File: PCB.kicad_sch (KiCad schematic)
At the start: 34 parts, among them J1 USB_C_Receptacle_USB2.0, J2 JST - 1.00mm 4 Pin, SW72 SW_Push, SW73 SW_Push, U1 RP2040, U2 SOP-8 SPI FLASH, U3 USBLC6-2SC6, U4 3.3V Fixed Regulator, Y1 12MHz Crystal 3225

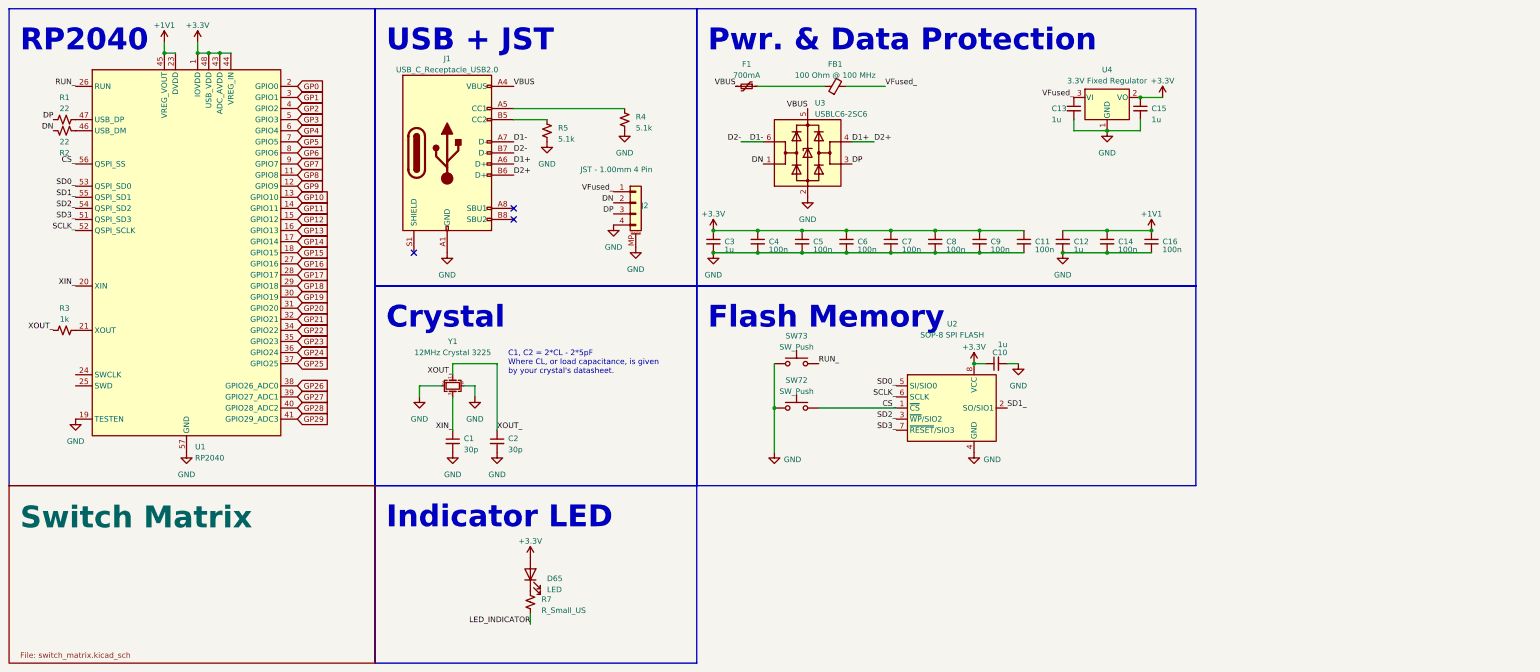
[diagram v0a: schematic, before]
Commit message: Layout complete
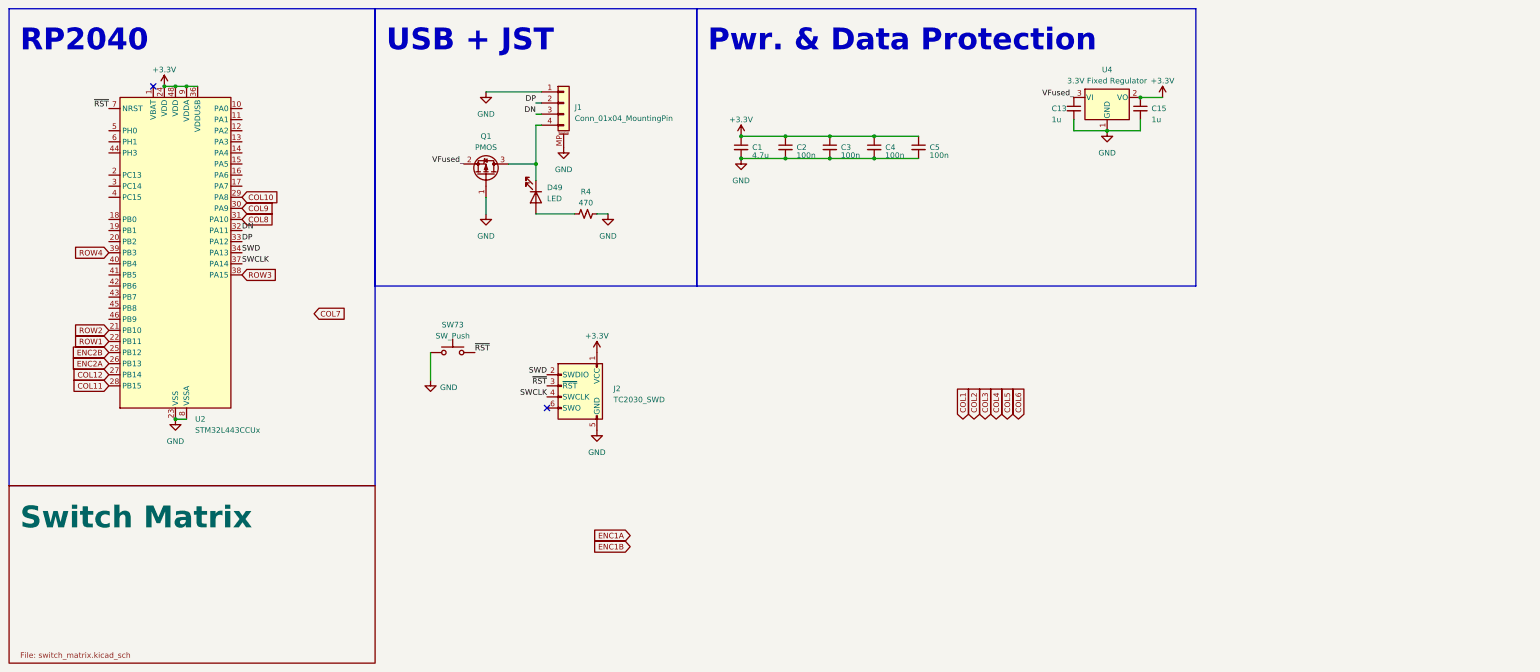
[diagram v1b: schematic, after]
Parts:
- removed C10, C12: 1u, Capacitor_SMD:C_0402_1005Metric, symbol Device:C_Small
- removed C11, C14, C16, C6, C7, C8, C9: 100n, Capacitor_SMD:C_0402_1005Metric, symbol Device:C_Small
- removed D65: LED, marbastlib-mx:LED_MX_3mm, symbol Device:LED
- removed F1: 700mA, Fuse:Fuse_0402_1005Metric, symbol Device:Polyfuse_Small
- removed FB1: 100 Ohm @ 100 MHz, Inductor_SMD:L_0402_1005Metric, symbol Device:FerriteBead_Small
- removed J1: USB_C_Receptacle_USB2.0, Connector_USB:USB_C_Receptacle_GCT_USB4085, symbol Connector:USB_C_Receptacle_USB2.0
- removed J2: JST - 1.00mm 4 Pin, Connector_JST:JST_SH_SM04B-SRSS-TB_1x04-1MP_P1.00mm_Horizontal, symbol Connector_Generic_MountingPin:Conn_01x04_MountingPin
- removed R1, R2: 22, Resistor_SMD:R_0402_1005Metric, symbol Device:R_Small_US
- removed R3: 1k, Resistor_SMD:R_0402_1005Metric, symbol Device:R_Small_US
- removed R5: 5.1k, Resistor_SMD:R_0402_1005Metric, symbol Device:R_Small_US
- removed R7: R_Small_US, Resistor_SMD:R_0402_1005Metric, symbol Device:R_Small_US
- removed SW72: SW_Push, Button_Switch_SMD:SW_SPST_SKQG_WithoutStem, symbol Switch:SW_Push
- removed U1: RP2040, Package_DFN_QFN:QFN-56-1EP_7x7mm_P0.4mm_EP3.2x3.2mm_ThermalVias, symbol MCU_RaspberryPi:RP2040
- removed U2: SOP-8 SPI FLASH, Package_SO:SOP-8_3.76x4.96mm_P1.27mm, symbol Memory_Flash:MX25R3235FZNxx0
- removed U3: USBLC6-2SC6, Package_TO_SOT_SMD:SOT-23-6, symbol Power_Protection:USBLC6-2SC6
- removed Y1: 12MHz Crystal 3225, Crystal:Crystal_SMD_3225-4Pin_3.2x2.5mm, symbol Device:Crystal_GND24_Small
- added D49: LED, Resistor_SMD:R_0603_1608Metric, symbol Device:LED
- added J1: Conn_01x04_MountingPin, Connector_Molex:Molex_Pico-EZmate_78171-0004_1x04-1MP_P1.20mm_Vertical, symbol Connector_Generic_MountingPin:Conn_01x04_MountingPin
- added J2: TC2030_SWD, PCM_marbastlib-various:CON_TC2030_outlined, symbol PCM_marbastlib-various:TC2030_SWD
- added Q1: PMOS, Package_TO_SOT_SMD:SOT-323_SC-70, symbol Device:Q_PMOS_GSD
- added U2: STM32L443CCUx, Package_DFN_QFN:QFN-48-1EP_7x7mm_P0.5mm_EP5.6x5.6mm_ThermalVias, symbol MCU_ST_STM32L4:STM32L443CCUx
- C1: value 30p -> 4.7u; LCSC C1562 -> C52923
- C2: value 30p -> 100n; LCSC C1562 -> C1525
- C3: value 1u -> 100n; LCSC C52923 -> C1525
- R4: value 5.1k -> 470; footprint Resistor_SMD:R_0402_1005Metric -> Resistor_SMD:R_0603_1608Metric; LCSC C25905 -> C23179
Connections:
- net XIN_ is gone; now on net +3.3V: C1.1
- net XOUT_ is gone; now on net +3.3V: C2.1
- net +3.3V: now also J2.1 (VCC), U2.24 (VDD), U2.36 (VDDUSB), U2.48 (VDD), U2.9 (VDDA)
- net DN: now also J1.3 (Pin_3), U2.32 (PA11)
- net DP: now also J1.2 (Pin_2), U2.33 (PA12)
- net GND: now also J1.1 (Pin_1), J1.MP (MountPin), J2.5 (GND), Q1.1 (G), U2.23 (VSS), U2.35 (VSS), U2.47 (VSS), U2.49 (VSS), U2.8 (VSSA)
- net VFused_: now also Q1.2 (S)
- net at R4.2: now also D49.2 (A)
- net RUN_ renamed ~{RST}
- net ~{RST}: now also J2.3 (~{RST}), U2.7 (NRST)
- new net: D49.1 (K), J1.4 (Pin_4), Q1.3 (D)
- new net COL10: U2.29 (PA8)
- new net COL11: U2.28 (PB15)
- new net COL12: U2.27 (PB14)
- new net COL8: U2.31 (PA10)
- new net COL9: U2.30 (PA9)
- new net ENC2A: U2.26 (PB13)
- new net ENC2B: U2.25 (PB12)
- new net ROW1: U2.22 (PB11)
- new net ROW2: U2.21 (PB10)
- new net ROW3: U2.38 (PA15)
- new net ROW4: U2.39 (PB3)
- new net SWCLK: J2.4 (SWCLK), U2.37 (PA14)
- new net SWD: J2.2 (SWDIO), U2.34 (PA13)
- no-connect marks 3 -> 2
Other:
- note removed: "C1, C2 = 2*CL - 2*5pF Where CL, or load capacitance, is given by your crystal's datasheet."
- note removed: "Crystal"
- note removed: "Flash Memory"
- note removed: "Indicator LED"
- moved on the sheet: SW73

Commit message: Revision most recent
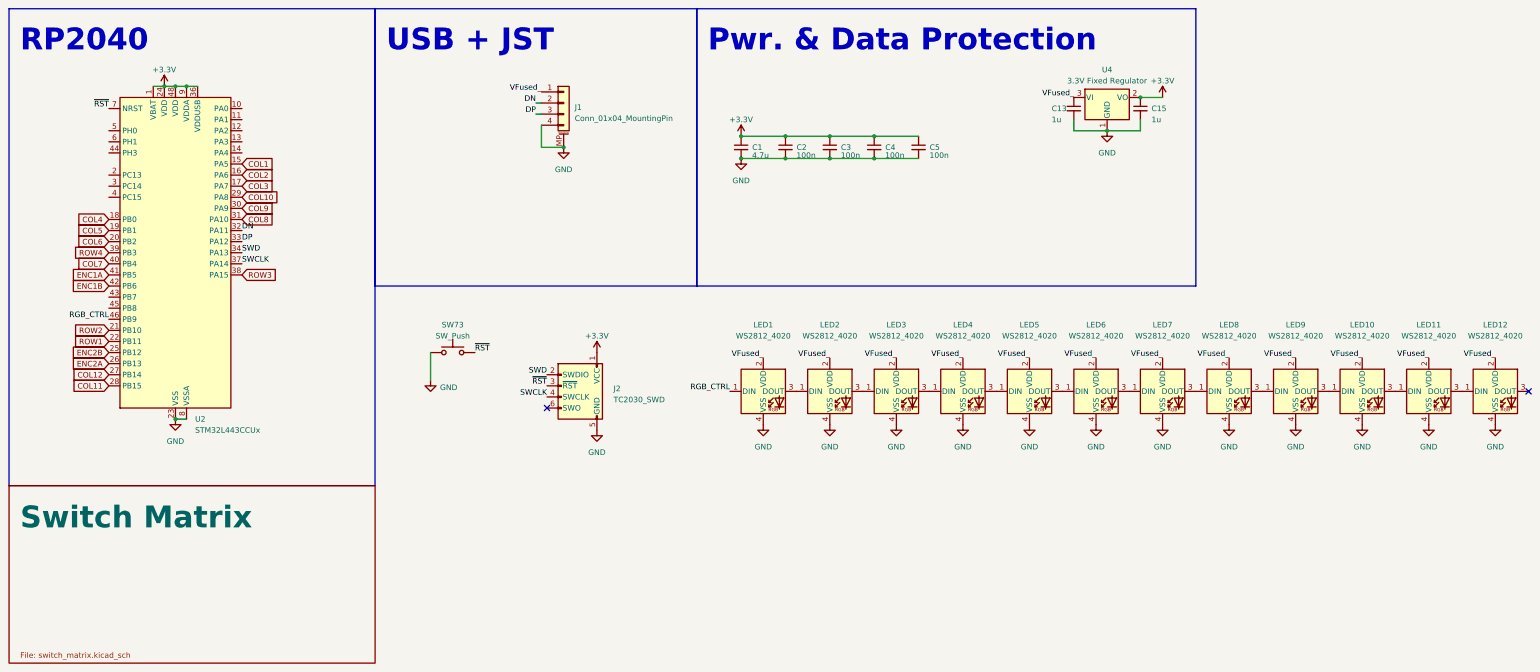
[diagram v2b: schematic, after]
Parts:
- removed D49: LED, Resistor_SMD:R_0603_1608Metric, symbol Device:LED
- removed Q1: PMOS, Package_TO_SOT_SMD:SOT-323_SC-70, symbol Device:Q_PMOS_GSD
- removed R4: 470, Resistor_SMD:R_0603_1608Metric, symbol Device:R_Small_US
- added LED1, LED10, LED11, LED12, LED2, LED3, LED4, LED5, LED6, LED7, LED8, LED9: WS2812_4020, PCM_marbastlib-various:LED_WS2812_4020, symbol marbastlib-various:WS2812_4020
- J1: footprint Connector_Molex:Molex_Pico-EZmate_78171-0004_1x04-1MP_P1.20mm_Vertical -> Connector_JST:JST_SH_SM04B-SRSS-TB_1x04-1MP_P1.00mm_Horizontal
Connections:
- net +3.3V: now also U2.1 (VBAT)
- net COL1: now also U2.15 (PA5)
- net COL2: now also U2.16 (PA6)
- net COL3: now also U2.17 (PA7)
- net COL4: now also U2.18 (PB0)
- net COL5: now also U2.19 (PB1)
- net COL6: now also U2.20 (PB2)
- net COL7: now also U2.40 (PB4)
- net DN: now also J1.2 (Pin_2); no longer J1.3 (Pin_3)
- net DP: now also J1.3 (Pin_3); no longer J1.2 (Pin_2)
- net ENC1A: now also U2.41 (PB5)
- net ENC1B: now also U2.42 (PB6)
- net GND: now also J1.4 (Pin_4), LED1.4 (VSS), LED10.4 (VSS), LED11.4 (VSS), LED12.4 (VSS), LED2.4 (VSS), LED3.4 (VSS), LED4.4 (VSS), LED5.4 (VSS), LED6.4 (VSS), LED7.4 (VSS), LED8.4 (VSS), LED9.4 (VSS); no longer J1.1 (Pin_1)
- net VFused_: now also J1.1 (Pin_1), LED1.2 (VDD), LED10.2 (VDD), LED11.2 (VDD), LED12.2 (VDD), LED2.2 (VDD), LED3.2 (VDD), LED4.2 (VDD), LED5.2 (VDD), LED6.2 (VDD), LED7.2 (VDD), LED8.2 (VDD), LED9.2 (VDD)
- net RGB_CTRL: now reaches U2.46 (PB9)
- net RGB_CTRL: now also LED1.1 (DIN)
- new net: LED10.1 (DIN), LED9.3 (DOUT)
- new net: LED10.3 (DOUT), LED11.1 (DIN)
- new net: LED3.3 (DOUT), LED4.1 (DIN)
- new net: LED4.3 (DOUT), LED5.1 (DIN)
- new net: LED6.3 (DOUT), LED7.1 (DIN)
- new net: LED7.3 (DOUT), LED8.1 (DIN)
- new net: LED1.3 (DOUT), LED2.1 (DIN)
- new net: LED2.3 (DOUT), LED3.1 (DIN)
- new net: LED8.3 (DOUT), LED9.1 (DIN)
- new net: LED5.3 (DOUT), LED6.1 (DIN)
- new net: LED11.3 (DOUT), LED12.1 (DIN)
